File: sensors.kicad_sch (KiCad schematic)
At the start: 3 parts, among them M4 Module-vr-max9924-0.1, M5 Module-knock-0.2, M6 Module-knock-0.2

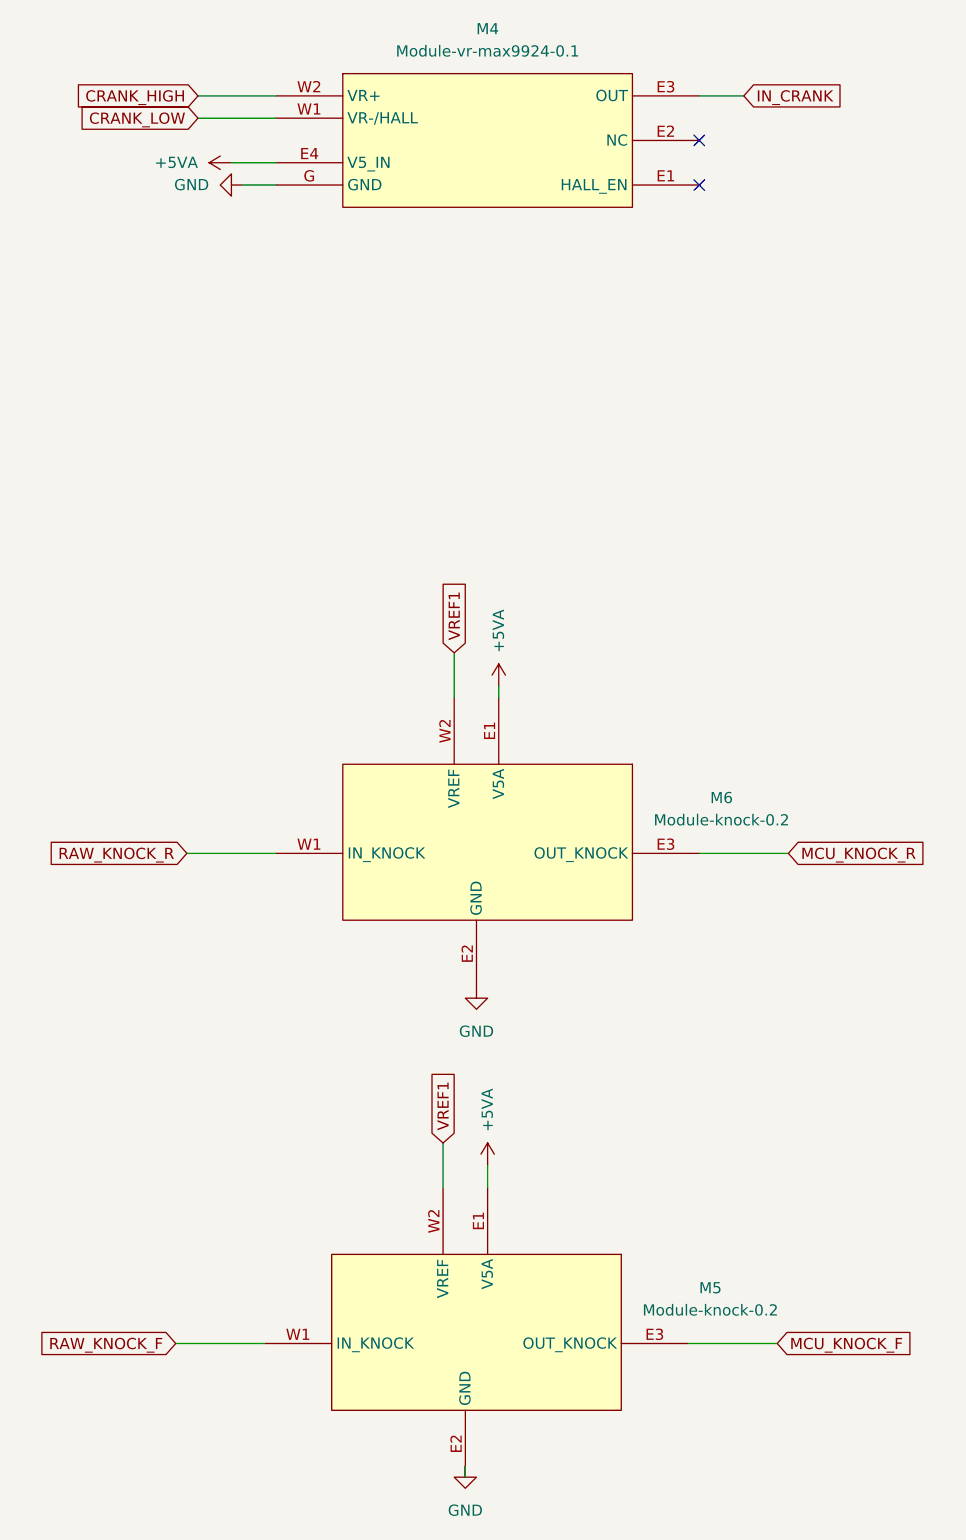
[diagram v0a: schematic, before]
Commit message: redone layout, possibly feature complete
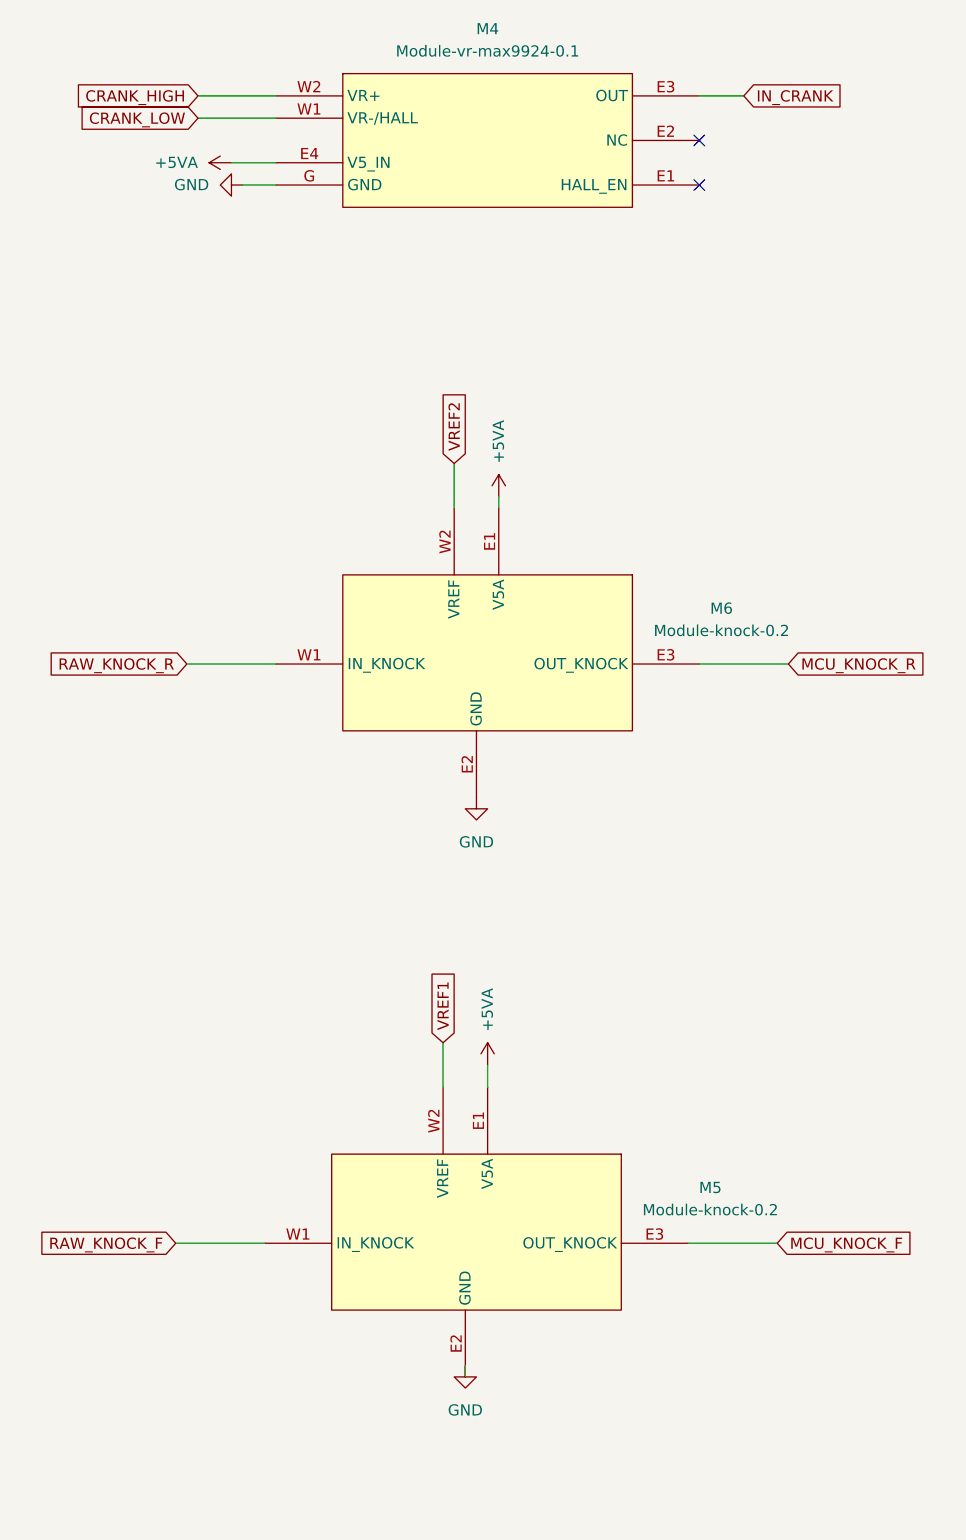
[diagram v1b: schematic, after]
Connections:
- net VREF1: no longer M6.W2 (VREF)
- new net VREF2: M6.W2 (VREF)
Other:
- moved on the sheet: M5, M6
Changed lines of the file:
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@@
 	(wire
 		(pts
-			(xy 90.17 118.11) (xy 100.33 118.11)
+			(xy 90.17 96.52) (xy 100.33 96.52)
 		)
 		(stroke
@@
 	(wire
 		(pts
-			(xy 60.96 151.13) (xy 60.96 156.21)
-		)
-		(stroke
-			(width 0)
-			(type default)
-		)
-	)
-	(wire
-		(pts
-			(xy 41.91 118.11) (xy 31.75 118.11)
+			(xy 60.96 139.7) (xy 60.96 144.78)
+		)
+		(stroke
+			(width 0)
+			(type default)
+		)
+	)
+	(wire
+		(pts
+			(xy 41.91 96.52) (xy 31.75 96.52)
 		)
 		(stroke
@@
 	(wire
 		(pts
-			(xy 40.64 173.99) (xy 30.48 173.99)
-		)
-		(stroke
-			(width 0)
-			(type default)
-		)
-	)
-	(wire
-		(pts
-			(xy 63.5 189.23) (xy 63.5 187.96)
-		)
-		(stroke
-			(width 0)
-			(type default)
-		)
-	)
-	(wire
-		(pts
-			(xy 67.31 100.33) (xy 67.31 99.06)
+			(xy 40.64 162.56) (xy 30.48 162.56)
+		)
+		(stroke
+			(width 0)
+			(type default)
+		)
+	)
+	(wire
+		(pts
+			(xy 63.5 177.8) (xy 63.5 176.53)
+		)
+		(stroke
+			(width 0)
+			(type default)
+		)
+	)
+	(wire
+		(pts
+			(xy 67.31 78.74) (xy 67.31 77.47)
 		)
 		(stroke
@@
 	(wire
 		(pts
-			(xy 62.23 95.25) (xy 62.23 100.33)
-		)
-		(stroke
-			(width 0)
-			(type default)
-		)
-	)
-	(wire
-		(pts
-			(xy 88.9 173.99) (xy 99.06 173.99)
-		)
-		(stroke
-			(width 0)
-			(type default)
-		)
-	)
-	(wire
-		(pts
-			(xy 66.04 156.21) (xy 66.04 153.67)
+			(xy 62.23 73.66) (xy 62.23 78.74)
+		)
+		(stroke
+			(width 0)
+			(type default)
+		)
+	)
+	(wire
+		(pts
+			(xy 88.9 162.56) (xy 99.06 162.56)
+		)
+		(stroke
+			(width 0)
+			(type default)
+		)
+	)
+	(wire
+		(pts
+			(xy 66.04 144.78) (xy 66.04 142.24)
 		)
 		(stroke
@@
 	(global_label "RAW_KNOCK_R"
 		(shape input)
-		(at 31.75 118.11 180)
+		(at 31.75 96.52 180)
 		(fields_autoplaced yes)
 		(effects
@@
 		)
 		(property "Intersheetrefs" "${INTERSHEET_REFS}"
-			(at 15.2786 118.11 0)
+			(at 15.2786 96.52 0)
 			(effects
 				(font
@@
 	(global_label "MCU_KNOCK_R"
 		(shape input)
-		(at 100.33 118.11 0)
+		(at 100.33 96.52 0)
 		(fields_autoplaced yes)
 		(effects
@@
 		)
 		(property "Intersheetrefs" "${INTERSHEET_REFS}"
-			(at 117.0433 118.11 0)
+			(at 117.0433 96.52 0)
 			(effects
 				(font
@@
 	(global_label "RAW_KNOCK_F"
 		(shape input)
-		(at 30.48 173.99 180)
+		(at 30.48 162.56 180)
 		(fields_autoplaced yes)
 		(effects
@@
 		)
 		(property "Intersheetrefs" "${INTERSHEET_REFS}"
-			(at 14.19 173.99 0)
+			(at 14.19 162.56 0)
 			(effects
 				(font
@@
 		)
 	)
-	(global_label "VREF1"
+	(global_label "VREF2"
 		(shape input)
-		(at 62.23 95.25 90)
+		(at 62.23 73.66 90)
 		(fields_autoplaced yes)
 		(effects
@@
 		)
 		(property "Intersheetrefs" "${INTERSHEET_REFS}"
-			(at 62.23 86.4591 90)
+			(at 62.23 64.8691 90)
 			(effects
 				(font
@@
 	(global_label "VREF1"
 		(shape input)
-		(at 60.96 151.13 90)
+		(at 60.96 139.7 90)
 		(fields_autoplaced yes)
 		(effects
@@
 		)
 		(property "Intersheetrefs" "${INTERSHEET_REFS}"
-			(at 60.96 142.3391 90)
+			(at 60.96 130.9091 90)
 			(effects
 				(font
@@
 	(global_label "MCU_KNOCK_F"
 		(shape input)
-		(at 99.06 173.99 0)
+		(at 99.06 162.56 0)
 		(fields_autoplaced yes)
 		(effects
@@
 		)
 		(property "Intersheetrefs" "${INTERSHEET_REFS}"
-			(at 115.5919 173.99 0)
+			(at 115.5919 162.56 0)
 			(effects
 				(font
@@
 	(symbol
 		(lib_id "power:+5VA")
-		(at 67.31 99.06 0)
+		(at 67.31 77.47 0)
 		(unit 1)
 		(exclude_from_sim no)
@@
 		(fields_autoplaced yes)
 		(property "Reference" "#PWR061"
-			(at 67.31 102.87 0)
+			(at 67.31 81.28 0)
 			(effects
 				(font
@@
 		)
 		(property "Value" "+5VA"
-			(at 67.3099 95.25 90)
+			(at 67.3099 73.66 90)
 			(effects
 				(font
@@
 		)
 		(property "Footprint" ""
-			(at 67.31 99.06 0)
+			(at 67.31 77.47 0)
 			(effects
 				(font
@@
 		)
 		(property "Datasheet" ""
-			(at 67.31 99.06 0)
+			(at 67.31 77.47 0)
 			(effects
 				(font
@@
 		)
 		(property "Description" "Power symbol creates a global label with name \"+5VA\""
-			(at 67.31 99.06 0)
+			(at 67.31 77.47 0)
 			(effects
 				(font
@@
 	(symbol
 		(lib_id "knock:Module-knock-0.2")
-		(at 48.26 163.83 0)
+		(at 48.26 152.4 0)
 		(unit 1)
 		(exclude_from_sim no)
@@
 		(fields_autoplaced yes)
 		(property "Reference" "M5"
-			(at 91.44 167.6714 0)
+			(at 91.44 156.2414 0)
 			(effects
 				(font
@@
 		)
 		(property "Value" "Module-knock-0.2"
-			(at 91.44 170.2114 0)
+			(at 91.44 158.7814 0)
 			(effects
 				(font
@@
 		)
 		(property "Footprint" "hellen_knock:knock"
-			(at 64.008 170.434 0)
+			(at 64.008 159.004 0)
 			(effects
 				(font
@@
 		)
 		(property "Datasheet" ""
-			(at 48.26 163.83 0)
+			(at 48.26 152.4 0)
 			(effects
 				(font
@@
 		)
 		(property "Description" "Hellen-One Knock Pre-amplifier Module"
-			(at 86.868 162.052 0)
+			(at 86.868 150.622 0)
 			(effects
 				(font
@@
 	(symbol
 		(lib_id "knock:Module-knock-0.2")
-		(at 49.53 107.95 0)
+		(at 49.53 86.36 0)
 		(unit 1)
 		(exclude_from_sim no)
@@
 		(fields_autoplaced yes)
 		(property "Reference" "M6"
-			(at 92.71 111.7914 0)
+			(at 92.71 90.2014 0)
 			(effects
 				(font
@@
 		)
 		(property "Value" "Module-knock-0.2"
-			(at 92.71 114.3314 0)
+			(at 92.71 92.7414 0)
 			(effects
 				(font
@@
 		)
 		(property "Footprint" "hellen_knock:knock"
-			(at 65.278 114.554 0)
+			(at 65.278 92.964 0)
 			(effects
 				(font
@@
 		)
 		(property "Datasheet" ""
-			(at 49.53 107.95 0)
+			(at 49.53 86.36 0)
 			(effects
 				(font
@@
 		)
 		(property "Description" "Hellen-One Knock Pre-amplifier Module"
-			(at 88.138 106.172 0)
+			(at 88.138 84.582 0)
 			(effects
 				(font
@@
 	(symbol
 		(lib_id "power:GND")
-		(at 64.77 133.35 0)
+		(at 64.77 111.76 0)
 		(unit 1)
 		(exclude_from_sim no)
@@
 		(fields_autoplaced yes)
 		(property "Reference" "#PWR046"
-			(at 64.77 139.7 0)
+			(at 64.77 118.11 0)
 			(effects
 				(font
@@
 		)
 		(property "Value" "GND"
-			(at 64.77 138.43 0)
+			(at 64.77 116.84 0)
 			(effects
 				(font
@@
 		)
 		(property "Footprint" ""
-			(at 64.77 133.35 0)
+			(at 64.77 111.76 0)
 			(effects
 				(font
@@
 		)
 		(property "Datasheet" ""
-			(at 64.77 133.35 0)
+			(at 64.77 111.76 0)
 			(effects
 				(font
@@
 		)
 		(property "Description" "Power symbol creates a global label with name \"GND\" , ground"
-			(at 64.77 133.35 0)
+			(at 64.77 111.76 0)
 			(effects
 				(font
@@
 	(symbol
 		(lib_id "power:GND")
-		(at 63.5 187.96 0)
+		(at 63.5 176.53 0)
 		(unit 1)
 		(exclude_from_sim no)
@@
 		(fields_autoplaced yes)
 		(property "Reference" "#PWR021"
-			(at 63.5 194.31 0)
+			(at 63.5 182.88 0)
 			(effects
 				(font
@@
 		)
 		(property "Value" "GND"
-			(at 63.5 193.04 0)
+			(at 63.5 181.61 0)
 			(effects
 				(font
@@
 		)
 		(property "Footprint" ""
-			(at 63.5 187.96 0)
+			(at 63.5 176.53 0)
 			(effects
 				(font
@@
 		)
 		(property "Datasheet" ""
-			(at 63.5 187.96 0)
+			(at 63.5 176.53 0)
 			(effects
 				(font
@@
 		)
 		(property "Description" "Power symbol creates a global label with name \"GND\" , ground"
-			(at 63.5 187.96 0)
+			(at 63.5 176.53 0)
 			(effects
 				(font
@@
 	(symbol
 		(lib_id "power:+5VA")
-		(at 66.04 153.67 0)
+		(at 66.04 142.24 0)
 		(unit 1)
 		(exclude_from_sim no)
@@
 		(fields_autoplaced yes)
 		(property "Reference" "#PWR062"
-			(at 66.04 157.48 0)
+			(at 66.04 146.05 0)
 			(effects
 				(font
@@
 		)
 		(property "Value" "+5VA"
-			(at 66.0399 149.86 90)
+			(at 66.0399 138.43 90)
 			(effects
 				(font
@@
 		)
 		(property "Footprint" ""
-			(at 66.04 153.67 0)
+			(at 66.04 142.24 0)
 			(effects
 				(font
@@
 		)
 		(property "Datasheet" ""
-			(at 66.04 153.67 0)
+			(at 66.04 142.24 0)
 			(effects
 				(font
@@
 		)
 		(property "Description" "Power symbol creates a global label with name \"+5VA\""
-			(at 66.04 153.67 0)
-			(effects
-				(font
+			(at 66.04 142.24 0)
+			(effects
+				(font
